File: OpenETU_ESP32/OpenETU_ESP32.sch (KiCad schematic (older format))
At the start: 11 parts, among them J1 Conn_01x02, U1 LM1117-3.3, U2 ESP32-PICO-D4

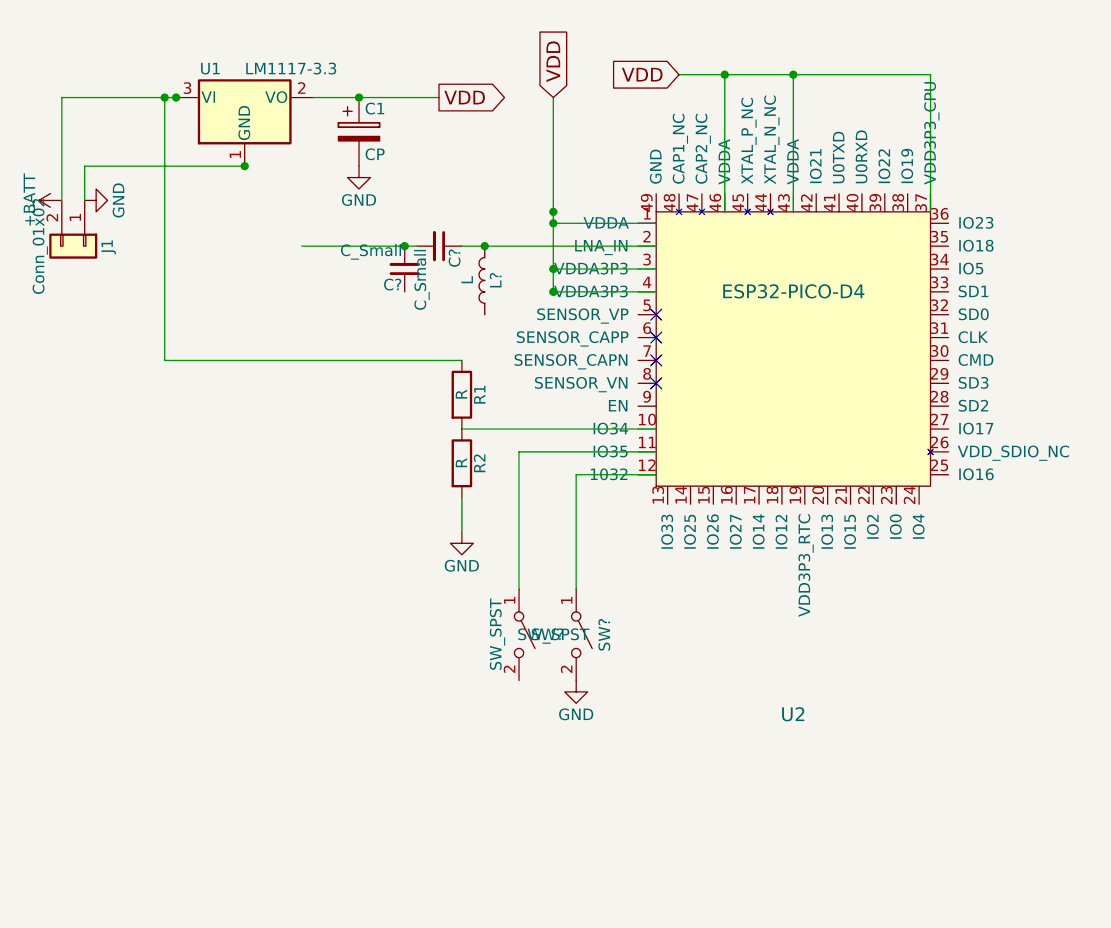
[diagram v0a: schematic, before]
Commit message: Just updating for the night
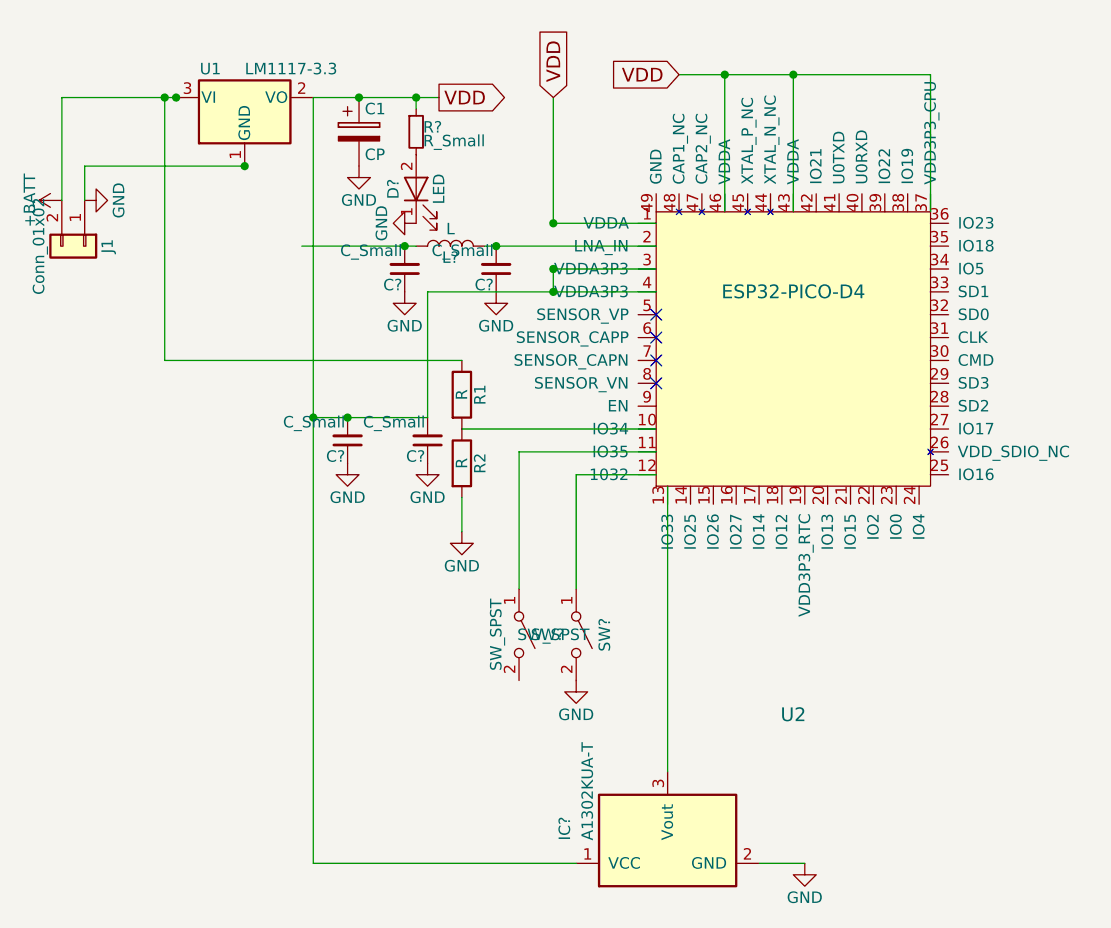
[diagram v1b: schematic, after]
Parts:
- added C? (x2): C_Small, symbol C_Small
- added D?: LED, symbol LED
- added IC?: A1302KUA-T, symbol A1302KUA-T
- added R?: R_Small, symbol R_Small
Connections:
- wire segments 23 -> 31
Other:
- moved on the sheet: C?, L?
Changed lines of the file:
@@
 LIBS:valves
 LIBS:esp32-pico-d4
+LIBS:ETrigger-smaliffying-cache
 LIBS:OpenETU_ESP32-cache
 EELAYER 25 0
@@
 	1    0    0    -1
 $EndComp
-Wire Wire Line
-	3650 2850 4200 2850
 $Comp
 L GND #PWR01
@@
 	1    0    0    -1
 $EndComp
-Connection ~ 3850 2850
 Text GLabel 4200 2850 2    60   Output ~ 0
 VDD
-Wire Wire Line
-	5150 3400 4700 3400
-Wire Wire Line
-	4700 2850 4700 3700
-Wire Wire Line
-	4700 3700 5150 3700
-Connection ~ 4700 3400
-Wire Wire Line
-	5150 3600 4700 3600
-Connection ~ 4700 3600
 Text GLabel 4700 2850 1    60   Input ~ 0
 VDD
-Wire Wire Line
-	5450 3350 5450 2750
-Wire Wire Line
-	5250 2750 6350 2750
-Wire Wire Line
-	5750 2750 5750 3350
-Wire Wire Line
-	6350 2750 6350 3350
-Connection ~ 5750 2750
-Connection ~ 5450 2750
 Text GLabel 5250 2750 0    60   Input ~ 0
 VDD
@@
 NoConn ~ 5150 4000
 NoConn ~ 5150 4100
-Wire Wire Line
-	3050 2850 2550 2850
-Wire Wire Line
-	2550 2850 2550 3300
 $Comp
 L Conn_01x02 J1
@@
 	0    1    1    0
 $EndComp
-Wire Wire Line
-	3350 3150 2650 3150
-Wire Wire Line
-	2650 3150 2650 3300
-Connection ~ 3000 2850
 $Comp
 L R R1
@@
 	1    0    0    -1
 $EndComp
-Wire Wire Line
-	3000 2850 3000 4000
-Wire Wire Line
-	3000 4000 4300 4000
-Wire Wire Line
-	4300 4300 5150 4300
 $Comp
 L R R2
@@
 	1    0    0    -1
 $EndComp
-Wire Wire Line
-	4300 4600 4300 4750
 $Comp
 L GND #PWR02
@@
 	0    -1   -1   0
 $EndComp
-Connection ~ 3350 3150
-Connection ~ 4700 3700
-Connection ~ 4700 3350
-Connection ~ 3050 2850
-Wire Wire Line
-	4300 3500 5150 3500
 $Comp
 L L L?
 U 1 1 5A060289
-P 4400 3650
-F 0 "L?" V 4350 3650 50  0000 C CNN
-F 1 "L" V 4475 3650 50  0000 C CNN
-F 2 "" H 4400 3650 50  0001 C CNN
-F 3 "" H 4400 3650 50  0001 C CNN
-	1    4400 3650
-	-1   0    0    1
+P 4250 3500
+F 0 "L?" V 4200 3500 50  0000 C CNN
+F 1 "L" V 4325 3500 50  0000 C CNN
+F 2 "" H 4250 3500 50  0001 C CNN
+F 3 "" H 4250 3500 50  0001 C CNN
+	1    4250 3500
+	0    -1   -1   0
 $EndComp
 $Comp
 L C_Small C?
 U 1 1 5A06032C
-P 4200 3500
-F 0 "C?" H 4210 3570 50  0000 L CNN
-F 1 "C_Small" H 4210 3420 50  0000 L CNN
-F 2 "" H 4200 3500 50  0001 C CNN
-F 3 "" H 4200 3500 50  0001 C CNN
-	1    4200 3500
-	0    1    1    0
-$EndComp
-Connection ~ 4400 3500
+P 4450 3600
+F 0 "C?" H 4460 3670 50  0000 L CNN
+F 1 "C_Small" H 4460 3520 50  0000 L CNN
+F 2 "" H 4450 3600 50  0001 C CNN
+F 3 "" H 4450 3600 50  0001 C CNN
+	1    4450 3600
+	-1   0    0    1
+$EndComp
 $Comp
 L C_Small C?
@@
 	-1   0    0    1
 $EndComp
-Wire Wire Line
-	3600 3500 4100 3500
-Connection ~ 4050 3500
-Wire Wire Line
-	5150 4400 4550 4400
-Wire Wire Line
-	4550 4400 4550 5000
 $Comp
 L SW_SPST SW?
@@
 	0    1    1    0
 $EndComp
-Wire Wire Line
-	5150 4500 4800 4500
-Wire Wire Line
-	4800 4500 4800 5000
 $Comp
 L GND #PWR?
@@
 	1    0    0    -1
 $EndComp
+$Comp
+L A1302KUA-T IC?
+U 1 1 5A067DC6
+P 5200 6100
+F 0 "IC?" H 5200 6550 50  0000 L CNN
+F 1 "A1302KUA-T" H 5200 6450 50  0000 L CNN
+F 2 "" H 5200 5750 50  0000 L CIN
+F 3 "" H 5100 6100 50  0000 C CNN
+	1    5200 6100
+	0    -1   -1   0
+$EndComp
+$Comp
+L R_Small R?
+U 1 1 5A06832A
+P 4100 3000
+F 0 "R?" H 4130 3020 50  0000 L CNN
+F 1 "R_Small" H 4130 2960 50  0000 L CNN
+F 2 "" H 4100 3000 50  0001 C CNN
+F 3 "" H 4100 3000 50  0001 C CNN
+	1    4100 3000
+	1    0    0    -1
+$EndComp
+$Comp
+L LED D?
+U 1 1 5A0683C3
+P 4100 3250
+F 0 "D?" H 4100 3350 50  0000 C CNN
+F 1 "LED" H 4100 3150 50  0000 C CNN
+F 2 "" H 4100 3250 50  0001 C CNN
+F 3 "" H 4100 3250 50  0001 C CNN
+	1    4100 3250
+	0    -1   -1   0
+$EndComp
+$Comp
+L GND #PWR?
+U 1 1 5A068443
+P 4100 3400
+F 0 "#PWR?" H 4100 3150 50  0001 C CNN
+F 1 "GND" H 4100 3250 50  0000 C CNN
+F 2 "" H 4100 3400 50  0001 C CNN
+F 3 "" H 4100 3400 50  0001 C CNN
+	1    4100 3400
+	0    1    1    0
+$EndComp
+$Comp
+L GND #PWR?
+U 1 1 5A068CD8
+P 5800 6200
+F 0 "#PWR?" H 5800 5950 50  0001 C CNN
+F 1 "GND" H 5800 6050 50  0000 C CNN
+F 2 "" H 5800 6200 50  0001 C CNN
+F 3 "" H 5800 6200 50  0001 C CNN
+	1    5800 6200
+	1    0    0    -1
+$EndComp
+$Comp
+L GND #PWR?
+U 1 1 5A069779
+P 4050 3700
+F 0 "#PWR?" H 4050 3450 50  0001 C CNN
+F 1 "GND" H 4050 3550 50  0000 C CNN
+F 2 "" H 4050 3700 50  0001 C CNN
+F 3 "" H 4050 3700 50  0001 C CNN
+	1    4050 3700
+	1    0    0    -1
+$EndComp
+$Comp
+L GND #PWR?
+U 1 1 5A0697AE
+P 4450 3700
+F 0 "#PWR?" H 4450 3450 50  0001 C CNN
+F 1 "GND" H 4450 3550 50  0000 C CNN
+F 2 "" H 4450 3700 50  0001 C CNN
+F 3 "" H 4450 3700 50  0001 C CNN
+	1    4450 3700
+	1    0    0    -1
+$EndComp
+Wire Wire Line
+	3650 2850 4200 2850
+Connection ~ 3850 2850
+Wire Wire Line
+	5150 3400 4700 3400
+Wire Wire Line
+	4150 3700 5150 3700
+Connection ~ 4700 3400
+Wire Wire Line
+	5150 3600 4700 3600
+Connection ~ 4700 3600
+Wire Wire Line
+	5450 3350 5450 2750
+Wire Wire Line
+	5250 2750 6350 2750
+Wire Wire Line
+	5750 2750 5750 3350
+Wire Wire Line
+	6350 2750 6350 3350
+Connection ~ 5750 2750
+Connection ~ 5450 2750
+Wire Wire Line
+	3050 2850 2550 2850
+Wire Wire Line
+	2550 2850 2550 3300
+Wire Wire Line
+	3350 3150 2650 3150
+Wire Wire Line
+	2650 3150 2650 3300
+Connection ~ 3000 2850
+Wire Wire Line
+	3000 2850 3000 4000
+Wire Wire Line
+	3000 4000 4300 4000
+Wire Wire Line
+	4300 4300 5150 4300
+Wire Wire Line
+	4300 4600 4300 4750
+Connection ~ 3350 3150
+Connection ~ 4700 3700
+Connection ~ 3050 2850
+Wire Wire Line
+	3600 3500 4100 3500
+Connection ~ 4050 3500
+Wire Wire Line
+	5150 4400 4550 4400
+Wire Wire Line
+	4550 4400 4550 5000
+Wire Wire Line
+	5150 4500 4800 4500
+Wire Wire Line
+	4800 4500 4800 5000
+Wire Wire Line
+	5200 4550 5200 5800
+Wire Wire Line
+	4100 2850 4100 2900
+Connection ~ 4100 2850
+Wire Wire Line
+	4800 6200 3650 6200
+Wire Wire Line
+	3650 6200 3650 2850
+Wire Wire Line
+	5600 6200 5800 6200
+Wire Wire Line
+	5150 3500 4400 3500
+Connection ~ 4450 3500
+Wire Wire Line
+	4700 3400 4700 2850
+Wire Wire Line
+	4700 3600 4700 3700
+Wire Wire Line
+	4150 4250 4150 3700
+$Comp
+L C_Small C?
+U 1 1 5A06AB7D
+P 4150 4350
+F 0 "C?" H 4160 4420 50  0000 L CNN
+F 1 "C_Small" H 4160 4270 50  0000 L CNN
+F 2 "" H 4150 4350 50  0001 C CNN
+F 3 "" H 4150 4350 50  0001 C CNN
+	1    4150 4350
+	-1   0    0    1
+$EndComp
+$Comp
+L C_Small C?
+U 1 1 5A06ABD8
+P 3800 4350
+F 0 "C?" H 3810 4420 50  0000 L CNN
+F 1 "C_Small" H 3810 4270 50  0000 L CNN
+F 2 "" H 3800 4350 50  0001 C CNN
+F 3 "" H 3800 4350 50  0001 C CNN
+	1    3800 4350
+	-1   0    0    1
+$EndComp
+Wire Wire Line
+	3650 4250 4150 4250
+Connection ~ 3650 4250
+Connection ~ 3800 4250
+$Comp
+L GND #PWR?
+U 1 1 5A06AD2D
+P 3800 4450
+F 0 "#PWR?" H 3800 4200 50  0001 C CNN
+F 1 "GND" H 3800 4300 50  0000 C CNN
+F 2 "" H 3800 4450 50  0001 C CNN
+F 3 "" H 3800 4450 50  0001 C CNN
+	1    3800 4450
+	1    0    0    -1
+$EndComp
+$Comp
+L GND #PWR?
+U 1 1 5A06AD68
+P 4150 4450
+F 0 "#PWR?" H 4150 4200 50  0001 C CNN
+F 1 "GND" H 4150 4300 50  0000 C CNN
+F 2 "" H 4150 4450 50  0001 C CNN
+F 3 "" H 4150 4450 50  0001 C CNN
+	1    4150 4450
+	1    0    0    -1
+$EndComp
